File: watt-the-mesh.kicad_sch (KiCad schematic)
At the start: 10 parts, among them U2 TPS61022RWUR

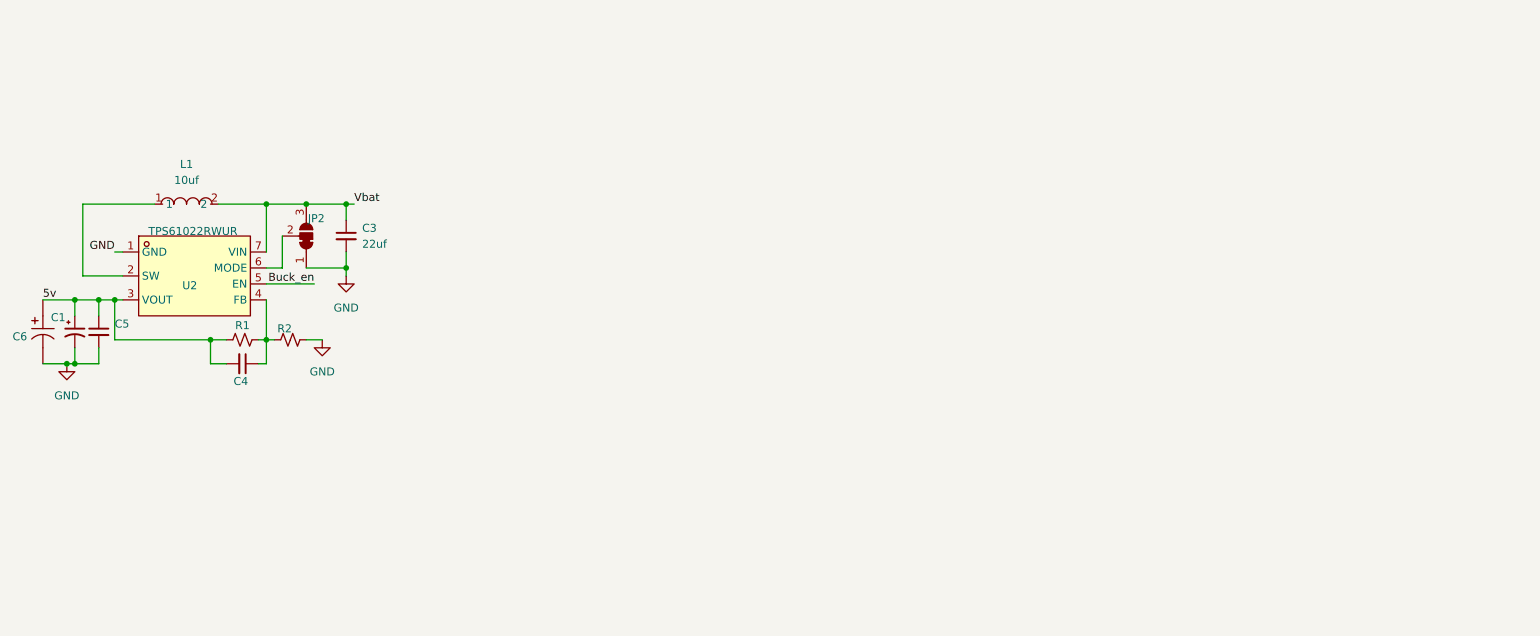
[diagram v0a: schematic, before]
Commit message: minor changes
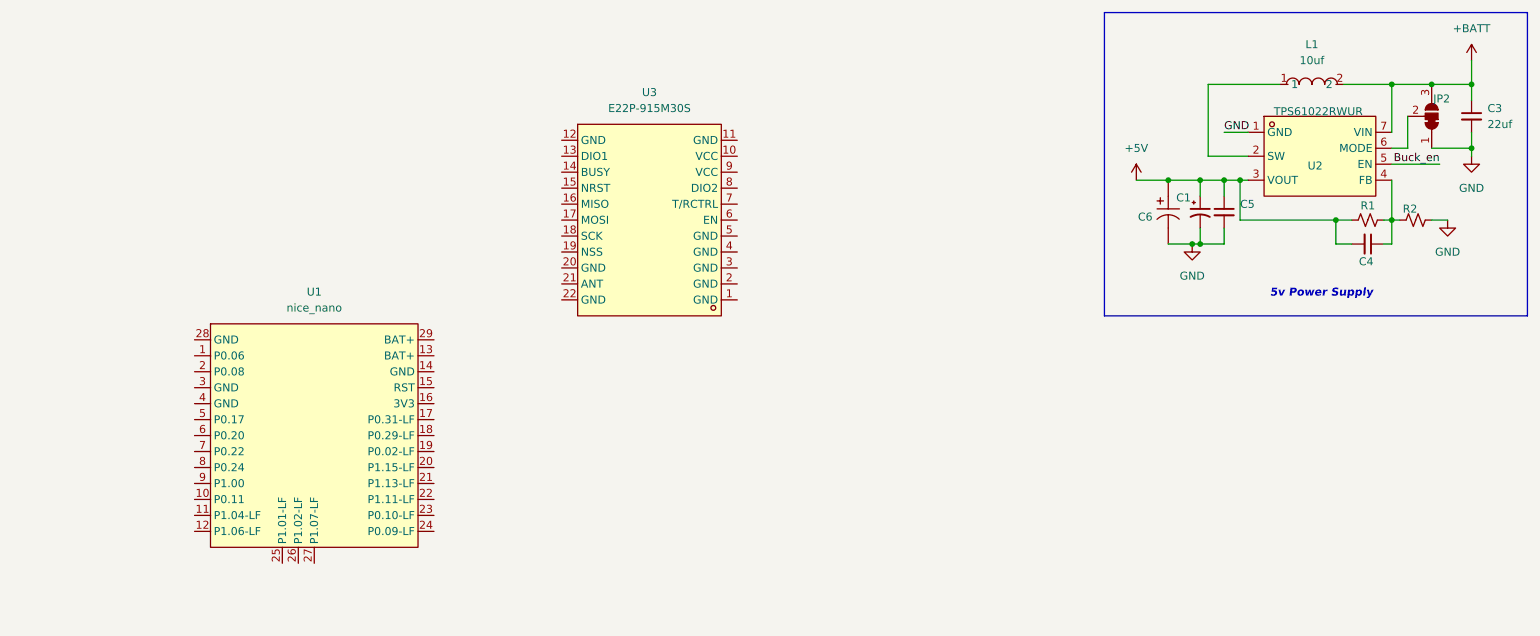
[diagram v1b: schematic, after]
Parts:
- added U1: nice_nano, PCM_marbastlib-xp-promicroish:nice_nano_AH_USBup, symbol PCM_marbastlib-promicroish:nice_nano
- added U3: E22P-915M30S, easyeda:COMM-SMD_22P-P2.54-L38.5-W24.0_E22-400M33S, symbol easyeda:E22P-915M30S
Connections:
- net 5v renamed +5V
- net Vbat renamed +BATT
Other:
- note added: "5v Power Supply"
- moved on the sheet: C1, C3, C4, C5, C6, JP2, L1, R1, R2, U2

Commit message: minor schematics changes
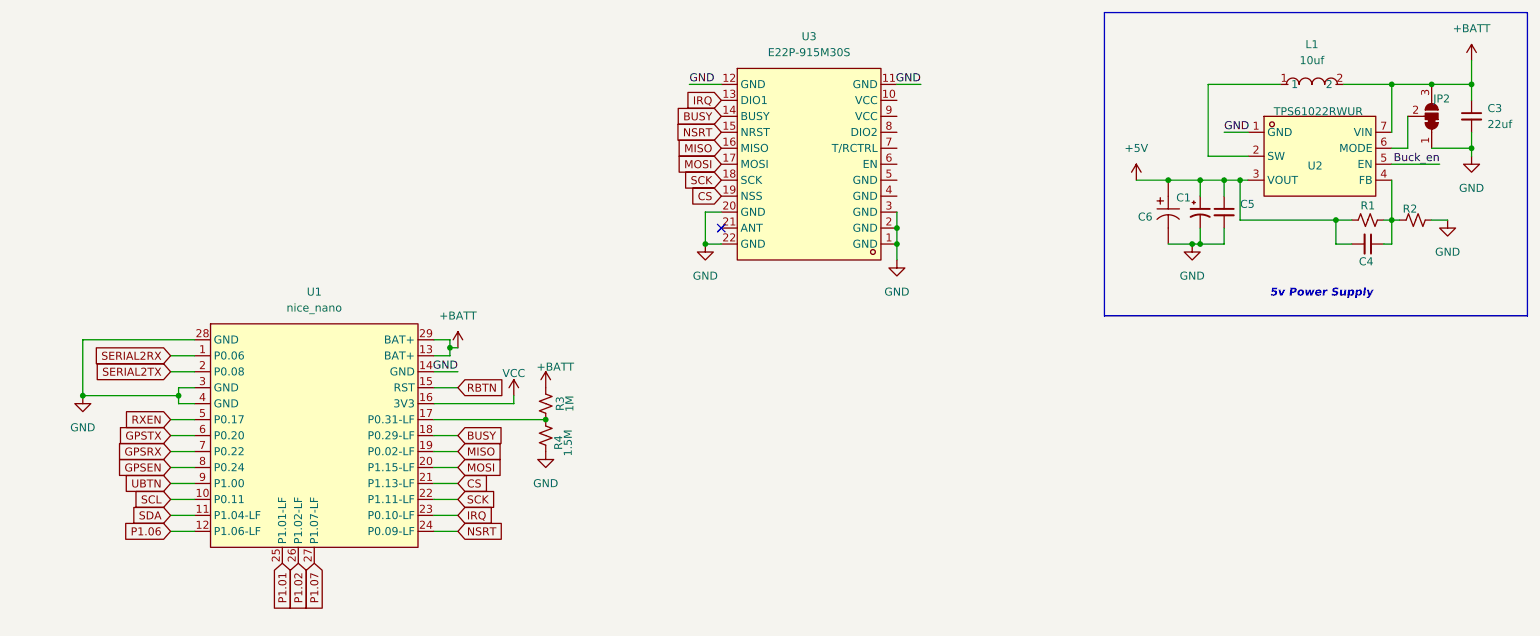
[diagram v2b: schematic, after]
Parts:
- added R3: 1M, Resistor_SMD:R_0603_1608Metric, symbol Device:R_Small_US
- added R4: 1.5M, Resistor_SMD:R_0603_1608Metric, symbol Device:R_Small_US
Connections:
- net +BATT: now also U1.13 (BAT+), U1.29 (BAT+), R3.2
- net GND: now also U1.14 (GND), U1.28 (GND), U1.3 (GND), U1.4 (GND), U3.1 (GND), U3.11 (GND), U3.12 (GND), U3.2 (GND), U3.20 (GND), U3.22 (GND), U3.3 (GND), R4.2
- net IRQ: now reaches U3.13 (DIO1)
- net IRQ: now also U1.23 (P0.10-LF)
- net BUSY: now reaches U3.14 (BUSY)
- net BUSY: now also U1.18 (P0.29-LF)
- net NSRT: now reaches U3.15 (NRST)
- net NSRT: now also U1.24 (P0.09-LF)
- net MISO: now reaches U3.16 (MISO)
- net MISO: now also U1.19 (P0.02-LF)
- net MOSI: now reaches U3.17 (MOSI)
- net MOSI: now also U1.20 (P1.15-LF)
- net SCK: now reaches U3.18 (SCK)
- net SCK: now also U1.22 (P1.11-LF)
- net CS: now reaches U3.19 (NSS)
- net CS: now also U1.21 (P1.13-LF)
- net SERIAL2RX: now reaches U1.1 (P0.06)
- net SCL: now reaches U1.10 (P0.11)
- net SDA: now reaches U1.11 (P1.04-LF)
- net P1.06: now reaches U1.12 (P1.06-LF)
- net RBTN: now reaches U1.15 (RST)
- net VCC: now reaches U1.16 (3V3)
- net at U1.17 (P0.31-LF): now also R3.1, R4.1
- net SERIAL2TX: now reaches U1.2 (P0.08)
- net P1.01: now reaches U1.25 (P1.01-LF)
- net P1.02: now reaches U1.26 (P1.02-LF)
- net P1.07: now reaches U1.27 (P1.07-LF)
- net RXEN: now reaches U1.5 (P0.17)
- net GPSTX: now reaches U1.6 (P0.20)
- net GPSRX: now reaches U1.7 (P0.22)
- net GPSEN: now reaches U1.8 (P0.24)
- net UBTN: now reaches U1.9 (P1.00)
- no-connect marks 0 -> 1
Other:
- moved on the sheet: U3
